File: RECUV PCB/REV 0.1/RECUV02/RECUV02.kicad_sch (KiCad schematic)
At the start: 15 parts, among them P1 VEXT, U1 ESP32-S3-WROOM-1, U2 CH340C

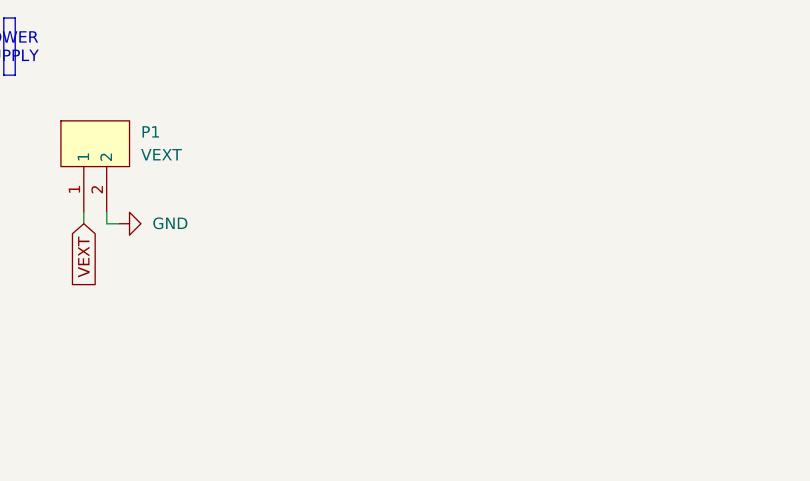
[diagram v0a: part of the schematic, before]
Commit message: added Schottky connection
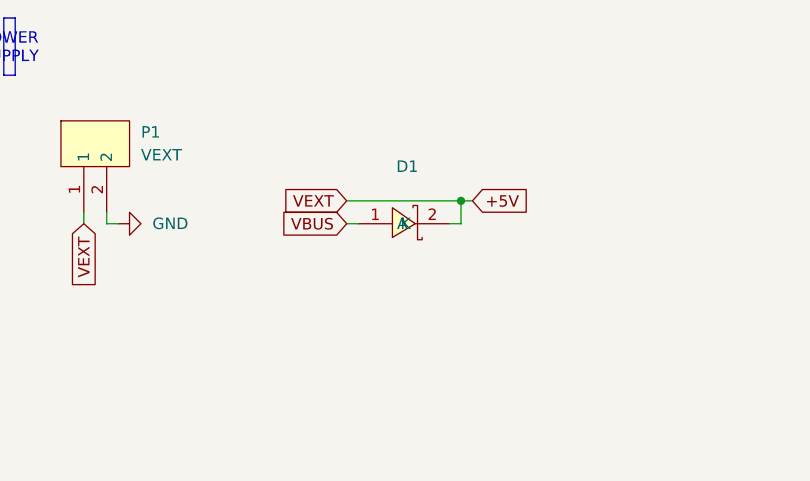
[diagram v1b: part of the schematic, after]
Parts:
- added D1: SS54_C22452, EasyEDA:SMA_L4.4-W2.8-LS5.4-R-RD, symbol EasyEDA:SS54_C22452
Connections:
- net VBUS: now also D1.1 (A)
- net VEXT renamed +5V
- net +5V: now also D1.2 (K)
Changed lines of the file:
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@@
+	)
+	(junction
+		(at 233.68 33.02)
+		(diameter 0)
+		(color 0 0 0 0)
 	)
 	(junction
@@
 	(wire
 		(pts
+			(xy 233.68 33.02) (xy 234.95 33.02)
+		)
+		(stroke
+			(width 0)
+			(type default)
+		)
+	)
+	(wire
+		(pts
 			(xy 68.58 36.83) (xy 69.85 36.83)
 		)
@@
 	(wire
 		(pts
+			(xy 220.98 33.02) (xy 233.68 33.02)
+		)
+		(stroke
+			(width 0)
+			(type default)
+		)
+	)
+	(wire
+		(pts
 			(xy 68.58 44.45) (xy 69.85 44.45)
 		)
@@
 	(wire
 		(pts
+			(xy 233.68 33.02) (xy 233.68 35.56)
+		)
+		(stroke
+			(width 0)
+			(type default)
+		)
+	)
+	(wire
+		(pts
 			(xy 119.38 54.61) (xy 113.03 54.61)
 		)
@@
 	(wire
 		(pts
+			(xy 232.41 35.56) (xy 233.68 35.56)
+		)
+		(stroke
+			(width 0)
+			(type default)
+		)
+	)
+	(wire
+		(pts
 			(xy 113.03 54.61) (xy 113.03 50.8)
 		)
@@
 		)
 	)
+	(wire
+		(pts
+			(xy 220.98 35.56) (xy 222.25 35.56)
+		)
+		(stroke
+			(width 0)
+			(type default)
+		)
+	)
 	(global_label "U0RXD"
 		(shape input)
@@
 		)
 	)
+	(global_label "VEXT"
+		(shape input)
+		(at 220.98 33.02 180)
+		(fields_autoplaced yes)
+		(effects
+			(font
+				(size 1.27 1.27)
+			)
+			(justify right)
+		)
+		(property "Intersheetrefs" "${INTERSHEET_REFS}"
+			(at 213.5801 33.02 0)
+			(hide yes)
+			(show_name no)
+			(do_not_autoplace no)
+			(effects
+				(font
+					(size 1.27 1.27)
+				)
+				(justify right)
+			)
+		)
+	)
 	(global_label "UD+"
 		(shape input)
@@
 		)
 	)
+	(global_label "+5V"
+		(shape input)
+		(at 234.95 33.02 0)
+		(fields_autoplaced yes)
+		(effects
+			(font
+				(size 1.27 1.27)
+			)
+			(justify left)
+		)
+		(property "Intersheetrefs" "${INTERSHEET_REFS}"
+			(at 241.8057 33.02 0)
+			(hide yes)
+			(show_name no)
+			(do_not_autoplace no)
+			(effects
+				(font
+					(size 1.27 1.27)
+				)
+				(justify left)
+			)
+		)
+	)
 	(global_label "UD-"
 		(shape input)
@@
 		(property "Intersheetrefs" "${INTERSHEET_REFS}"
 			(at 96.4377 54.61 0)
+			(hide yes)
+			(show_name no)
+			(do_not_autoplace no)
+			(effects
+				(font
+					(size 1.27 1.27)
+				)
+				(justify right)
+			)
+		)
+	)
+	(global_label "VBUS"
+		(shape input)
+		(at 220.98 35.56 180)
+		(fields_autoplaced yes)
+		(effects
+			(font
+				(size 1.27 1.27)
+			)
+			(justify right)
+		)
+		(property "Intersheetrefs" "${INTERSHEET_REFS}"
+			(at 213.0962 35.56 0)
 			(hide yes)
 			(show_name no)
@@
 					(unit 1)
 				)
+			)
+		)
+	)
+	(symbol
+		(lib_id "EasyEDA:SS54_C22452")
+		(at 227.33 35.56 180)
+		(unit 1)
+		(body_style 1)
+		(exclude_from_sim no)
+		(in_bom yes)
+		(on_board yes)
+		(in_pos_files yes)
+		(dnp no)
+		(fields_autoplaced yes)
+		(property "Reference" "D1"
+			(at 227.71 29.21 0)
+			(show_name no)
+			(do_not_autoplace no)
+			(effects
+				(font
+					(size 1.27 1.27)
+				)
+			)
+		)
+		(property "Value" "SS54_C22452"
+			(at 227.71 31.75 0)
+			(hide yes)
+			(show_name no)
+			(do_not_autoplace no)
+			(effects
+				(font
+					(size 1.27 1.27)
+				)
+			)
+		)
+		(property "Footprint" "EasyEDA:SMA_L4.4-W2.8-LS5.4-R-RD"
+			(at 227.33 27.94 0)
+			(hide yes)
+			(show_name no)
+			(do_not_autoplace no)
+			(effects
+				(font
+					(size 1.27 1.27)
+				)
+			)
+		)
+		(property "Datasheet" "https://lcsc.com/product-detail/Schottky-Barrier-Diodes-SBD_SS54_C22452.html"
+			(at 227.33 25.4 0)
+			(hide yes)
+			(show_name no)
+			(do_not_autoplace no)
+			(effects
+				(font
+					(size 1.27 1.27)
+				)
+			)
+		)
+		(property "Description" "SS54"
+			(at 227.33 35.56 0)
+			(hide yes)
+			(show_name no)
+			(do_not_autoplace no)
+			(effects
+				(font
+					(size 1.27 1.27)
+				)
+			)
+		)
+		(property "Manufacturer" "MDD(辰达半导体)"
+			(at 227.33 22.86 0)
+			(hide yes)
+			(show_name no)
+			(do_not_autoplace no)
+			(effects
+				(font
+					(size 1.27 1.27)
+				)
+			)
+		)
+		(property "MPN" "SS54"
+			(at 227.33 20.32 0)
+			(hide yes)
+			(show_name no)
+			(do_not_autoplace no)
+			(effects
+				(font
+					(size 1.27 1.27)
+				)
+			)
+		)
+		(property "LCSC Part" "C22452"
+			(at 227.33 17.78 0)
+			(hide yes)
+			(show_name no)
+			(do_not_autoplace no)
+			(effects
+				(font
+					(size 1.27 1.27)
+				)
+			)
+		)
+		(pin "2"
+		)
+		(pin "1"
+		)
+		(instances
+			(project "RECUV02"
+				(path "/2b6cdc4d-a2c2-48c0-8972-6d5f3f53de15"
+					(reference "D1")
+					(unit 1)
+				)
